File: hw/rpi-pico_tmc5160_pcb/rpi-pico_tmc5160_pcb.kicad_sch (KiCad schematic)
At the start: 9 parts, among them J1 Conn_01x04, J2 Conn_01x03, J3 Conn_01x04, J4 Conn_01x04, J5 Conn_01x04, U1 Pico

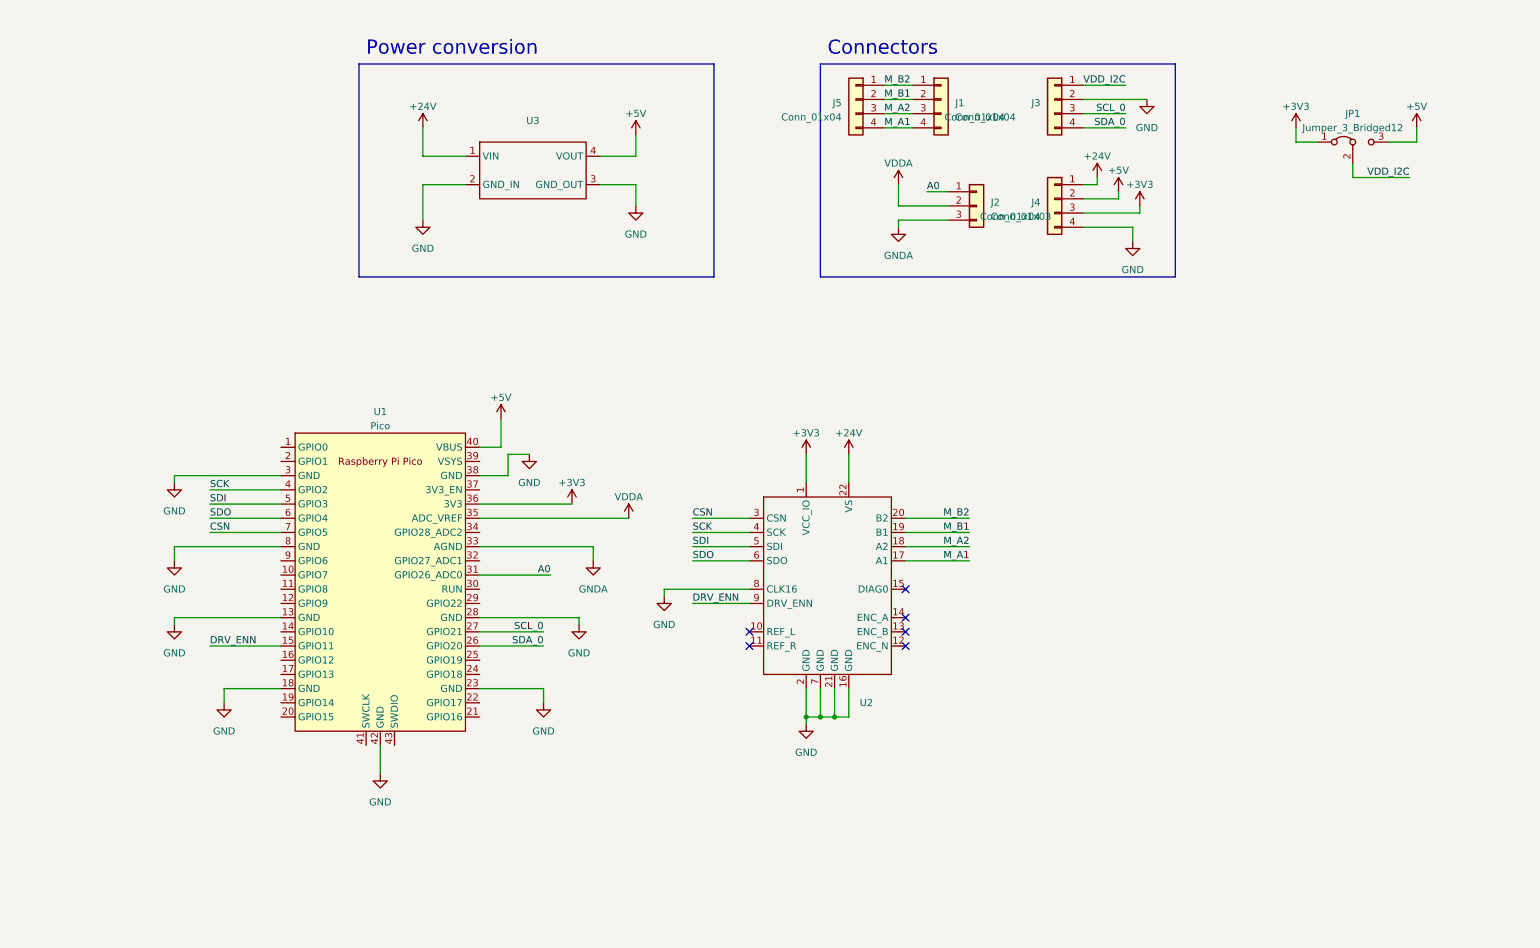
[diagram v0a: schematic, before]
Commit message: first PCB layout
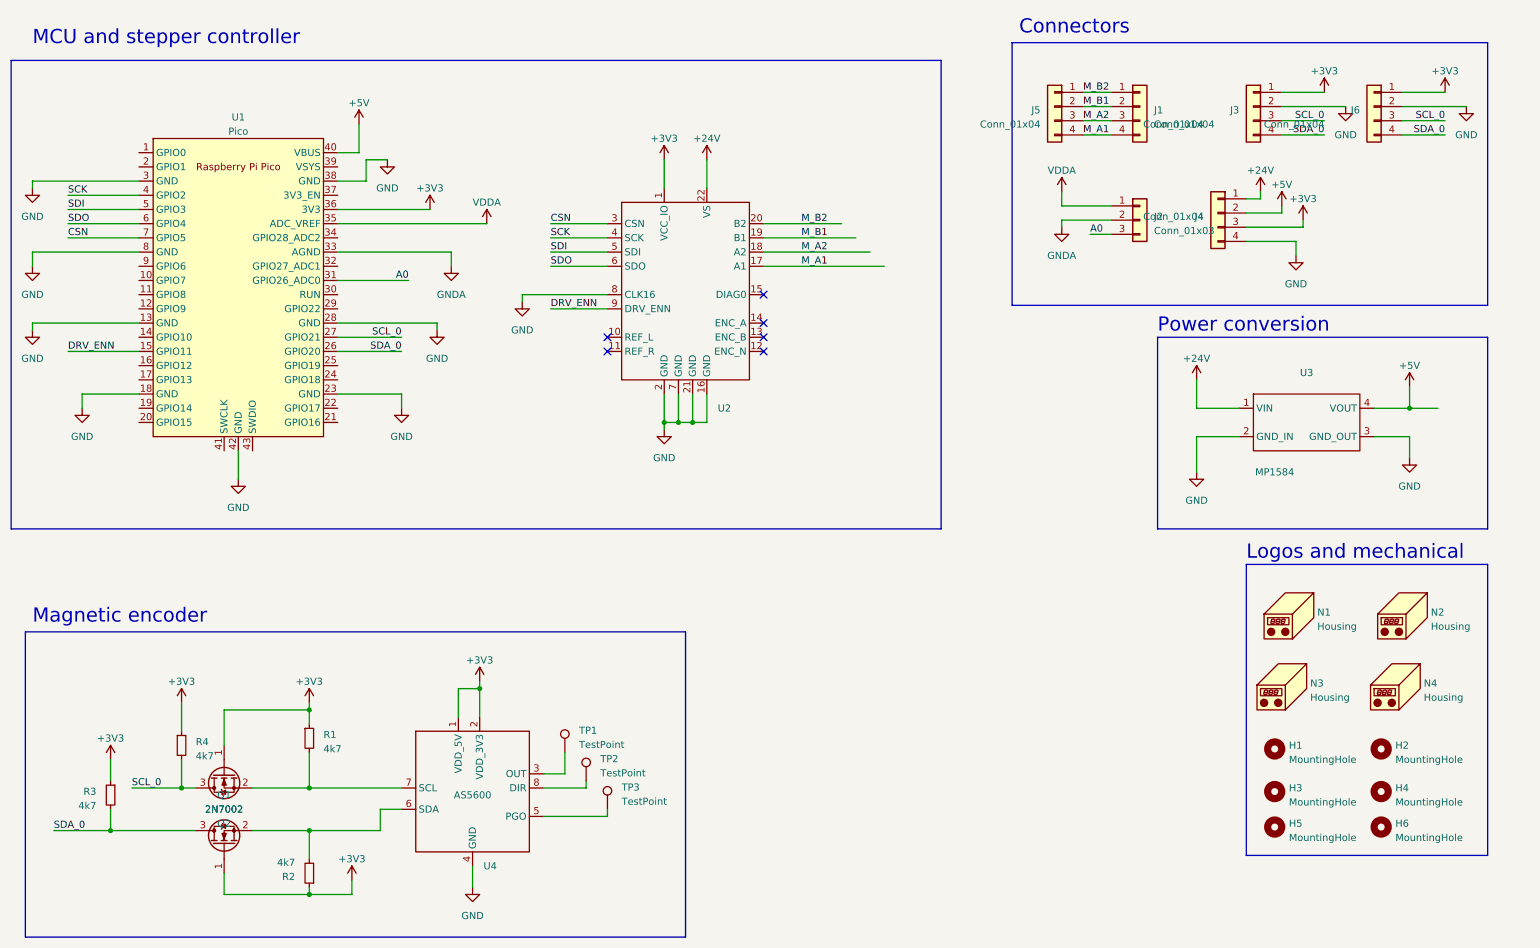
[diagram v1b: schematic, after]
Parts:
- removed JP1: Jumper_3_Bridged12, Jumper:SolderJumper-3_P1.3mm_Bridged12_RoundedPad1.0x1.5mm, symbol Jumper:Jumper_3_Bridged12
- added H1, H2, H3, H4, H5, H6: MountingHole, MountingHole:MountingHole_3.2mm_M3_ISO7380, symbol Mechanical:MountingHole
- added J6: Conn_01x04, Connector_JST:JST_XH_B4B-XH-A_1x04_P2.50mm_Vertical, symbol Connector_Generic:Conn_01x04
- added N1, N2, N3, N4: Housing, project:Mousebite, symbol Mechanical:Housing
- added Q1, Q2: 2N7002, Package_TO_SOT_SMD:SOT-23, symbol Transistor_FET:2N7002
- added R1, R2, R3, R4: 4k7, Resistor_SMD:R_0603_1608Metric_Pad0.98x0.95mm_HandSolder, symbol Device:R_Small
- added TP1, TP2, TP3: TestPoint, TestPoint:TestPoint_THTPad_2.0x2.0mm_Drill1.0mm, symbol Connector:TestPoint
- added U4: AS5600, Package_SO:SOIC-8_3.9x4.9mm_P1.27mm, symbol project_lib:AS5600
- J3, J5: footprint Connector_JST:JST_XH_B4B-XH-AM_1x04_P2.50mm_Vertical -> Connector_JST:JST_XH_B4B-XH-A_1x04_P2.50mm_Vertical
- U3: value ~ -> MP1584
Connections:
- net VDD_I2C is gone; now on net +3V3: J3.1 (Pin_1)
- net +3V3: now also J6.1 (Pin_1), Q1.1 (G), Q2.1 (G), R1.1, R2.1, R3.1, R4.1, U4.1 (VDD_5V), U4.2 (VDD_3V3)
- net A0: now also J2.3 (Pin_3); no longer J2.1 (Pin_1)
- net GND: now also J6.2 (Pin_2), U4.4 (GND)
- net GNDA: now also J2.2 (Pin_2); no longer J2.3 (Pin_3)
- net SCL_0: now also J6.3 (Pin_3), Q2.3 (D), R4.2
- net SDA_0: now also J6.4 (Pin_4), Q1.3 (D), R3.2
- net VDDA: now also J2.1 (Pin_1); no longer J2.2 (Pin_2)
- new net: TP3.1, U4.5 (PGO)
- new net: Q2.2 (S), R1.2, U4.7 (SCL)
- new net: TP1.1, U4.3 (OUT)
- new net: Q1.2 (S), R2.2, U4.6 (SDA)
- new net: TP2.1, U4.8 (DIR)
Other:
- note added: "Logos and mechanical"
- note added: "MCU and stepper controller"
- note added: "Magnetic encoder"
- title: (none) -> RPi-Pico_TMC5160
- moved on the sheet: J1, J2, J3, J4, J5, U1, U2, U3
